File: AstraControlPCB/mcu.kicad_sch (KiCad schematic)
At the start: 9 parts, among them U1 ESP32-S3-WROOM-1U-N8

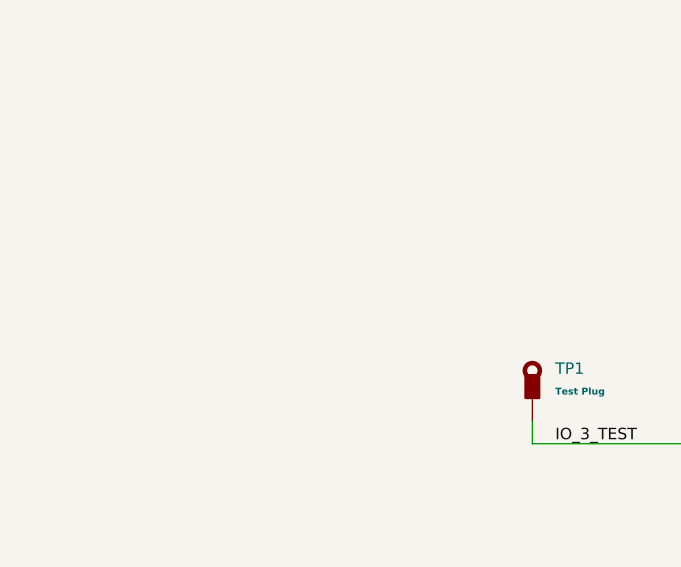
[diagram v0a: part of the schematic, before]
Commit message: Cleanup
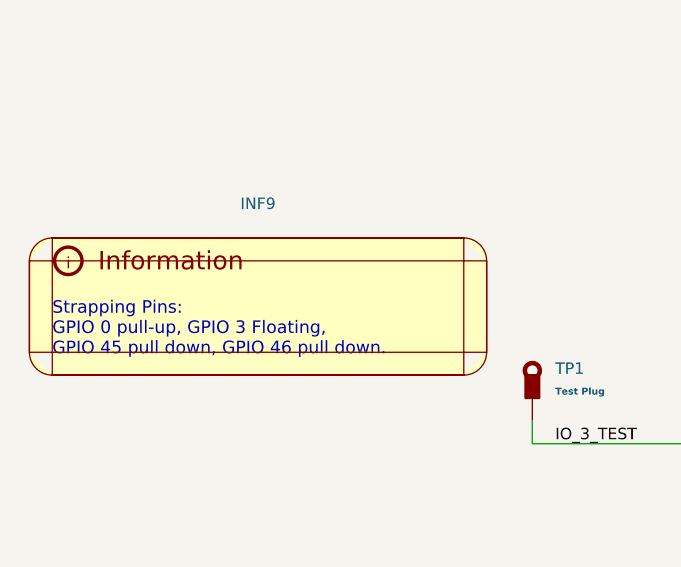
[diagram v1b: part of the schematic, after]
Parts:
- added INF9: ~, symbol LiveAstra:Information_Box
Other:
- note added: "Strapping Pins: GPIO 0 pull-up, GPIO 3 Floating, GPIO 45 pull down, GPIO 46 pull down."
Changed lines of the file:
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@@
+		)
+	)
+	(text "Strapping Pins: \nGPIO 0 pull-up, GPIO 3 Floating,\nGPIO 45 pull down, GPIO 46 pull down.\n"
+		(exclude_from_sim no)
+		(at 22.86 104.14 0)
+		(effects
+			(font
+				(face "ING Me")
+				(size 1.397 1.397)
+			)
+			(justify left)
 		)
 	)
@@
 					(unit 1)
 				)
+			)
+		)
+	)
+	(symbol
+		(lib_id "LiveAstra:Information_Box")
+		(at 45.72 101.6 0)
+		(unit 1)
+		(exclude_from_sim yes)
+		(in_bom no)
+		(on_board no)
+		(dnp no)
+		(fields_autoplaced yes)
+		(property "Reference" "INF9"
+			(at 45.72 90.17 0)
+			(effects
+				(font
+					(size 1.27 1.27)
+				)
+			)
+		)
+		(property "Value" "~"
+			(at 45.72 92.71 0)
+			(effects
+				(font
+					(size 1.27 1.27)
+				)
+			)
+		)
+		(property "Footprint" ""
+			(at 30.48 97.79 0)
+			(effects
+				(font
+					(size 1.27 1.27)
+				)
+				(hide yes)
+			)
+		)
+		(property "Datasheet" ""
+			(at 30.48 97.79 0)
+			(effects
+				(font
+					(size 1.27 1.27)
+				)
+				(hide yes)
+			)
+		)
+		(property "Description" ""
+			(at 30.48 97.79 0)
+			(effects
+				(font
+					(size 1.27 1.27)
+				)
+				(hide yes)
+			)
+		)
+		(instances
+			(project "AstraControl"
+				(path "/9a751838-dce8-4d69-8a02-736625ac74e7/0db21d8e-3390-4d67-877f-0e5d98e37848/3087dd4a-2a8a-4df4-b1d8-8d4a2b3256a2"
+					(reference "INF9")
+					(unit 1)
+				)
